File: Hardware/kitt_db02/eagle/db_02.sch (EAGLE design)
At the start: 30 parts, among them T8.1 TPTP09SQ, T8.2 TPTP09SQ, U8.0 MCP23017ML, X8.01 FTS-109-01-L-DV

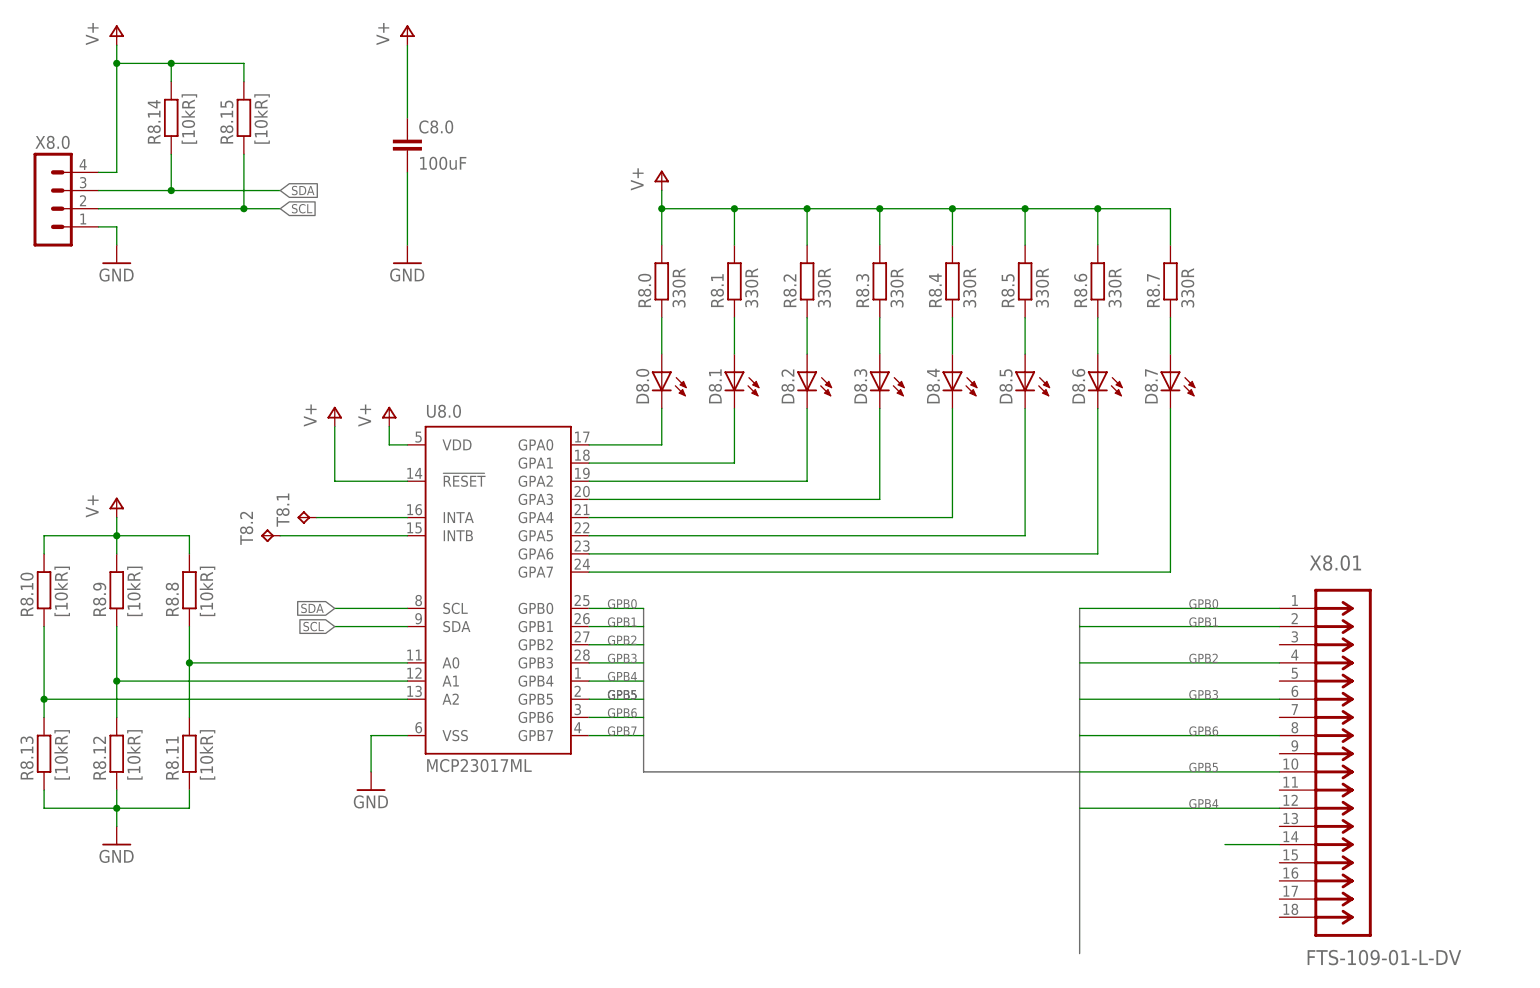
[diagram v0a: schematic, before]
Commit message: restored db02 board layout from commit acb6896f0427ddee216c2485e595b1a3f3064529
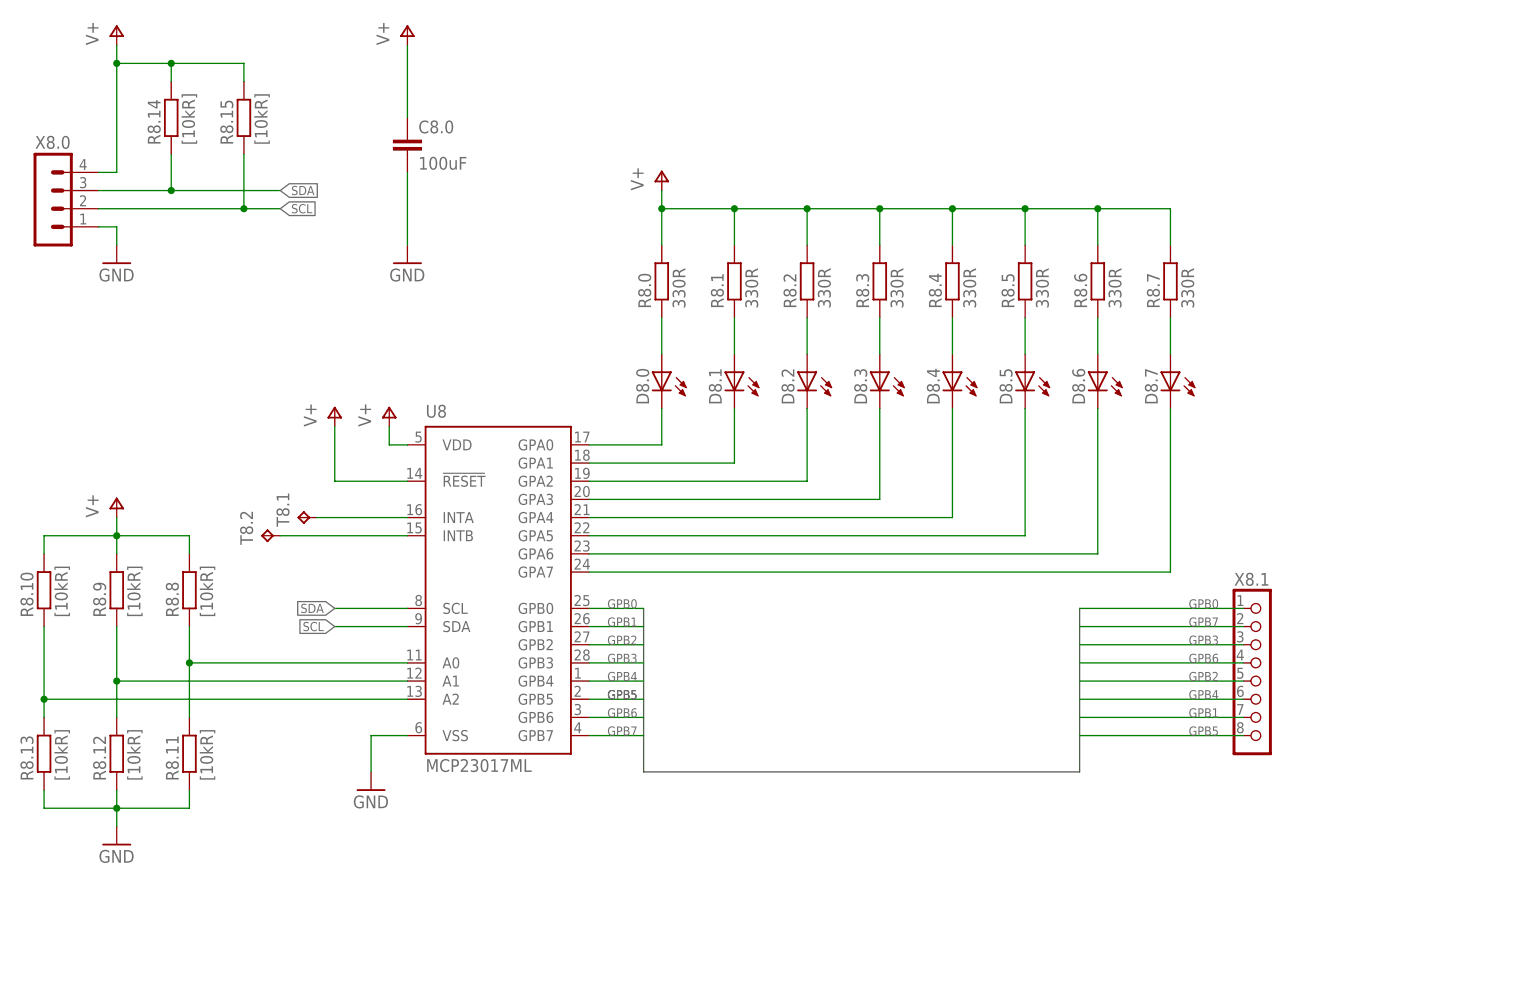
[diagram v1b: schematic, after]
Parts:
- removed X8.01: FTS-109-01-L-DV, kitt.con:FTS-109-01-L-DV
- added X8.1: CON_HEADER_1X08-SMD, dp_devices:CON_HEADER_1X08-SMD
- renumbered U8.0 to U8
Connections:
- net GPB0: now also X8.1.1; no longer X8.01.1
- net GPB1: now also X8.1.7; no longer X8.01.2
- net GPB2: now also X8.1.5; no longer X8.01.4
- net GPB3: now also X8.1.3; no longer X8.01.6
- net GPB4: now also X8.1.6; no longer X8.01.12
- net GPB5: now also X8.1.8; no longer X8.01.10
- net GPB6: now also X8.1.4; no longer X8.01.8
- net GPB7: now also X8.1.2; no longer X8.01.14
